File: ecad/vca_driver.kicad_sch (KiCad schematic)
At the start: 7 parts, among them Q2 BD140, Q4 BD139, U3 OPA2277

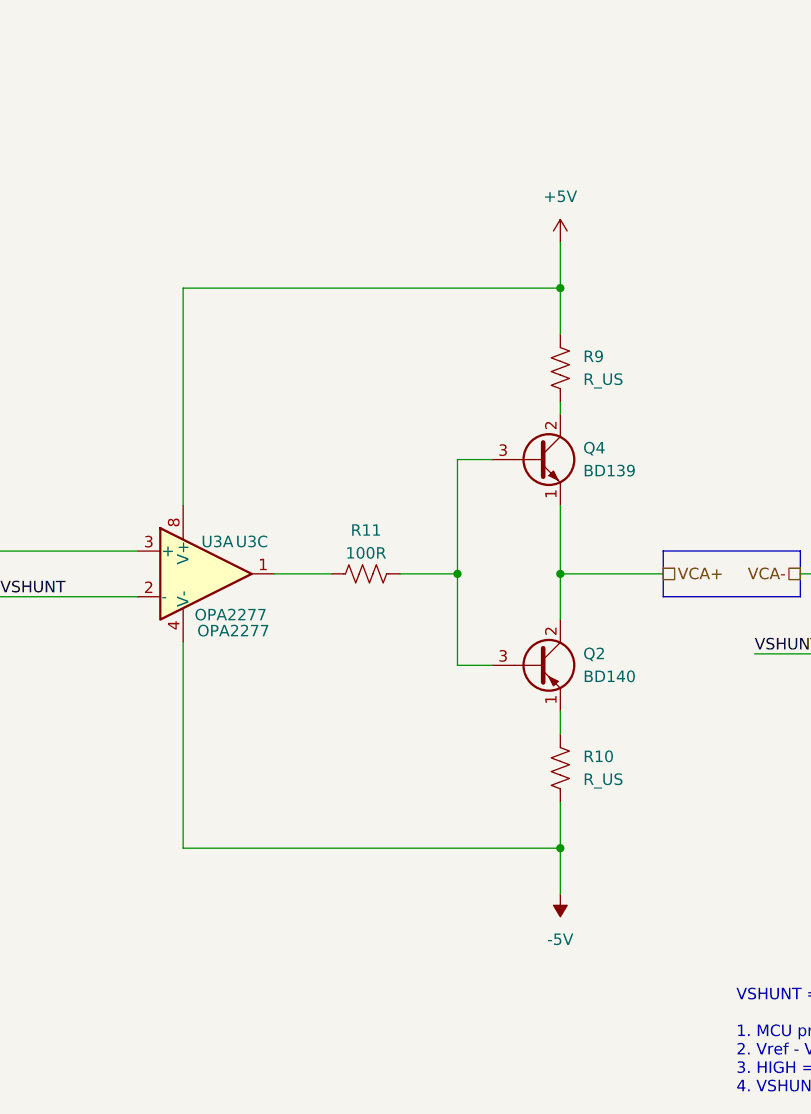
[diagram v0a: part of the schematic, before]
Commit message: more sizing
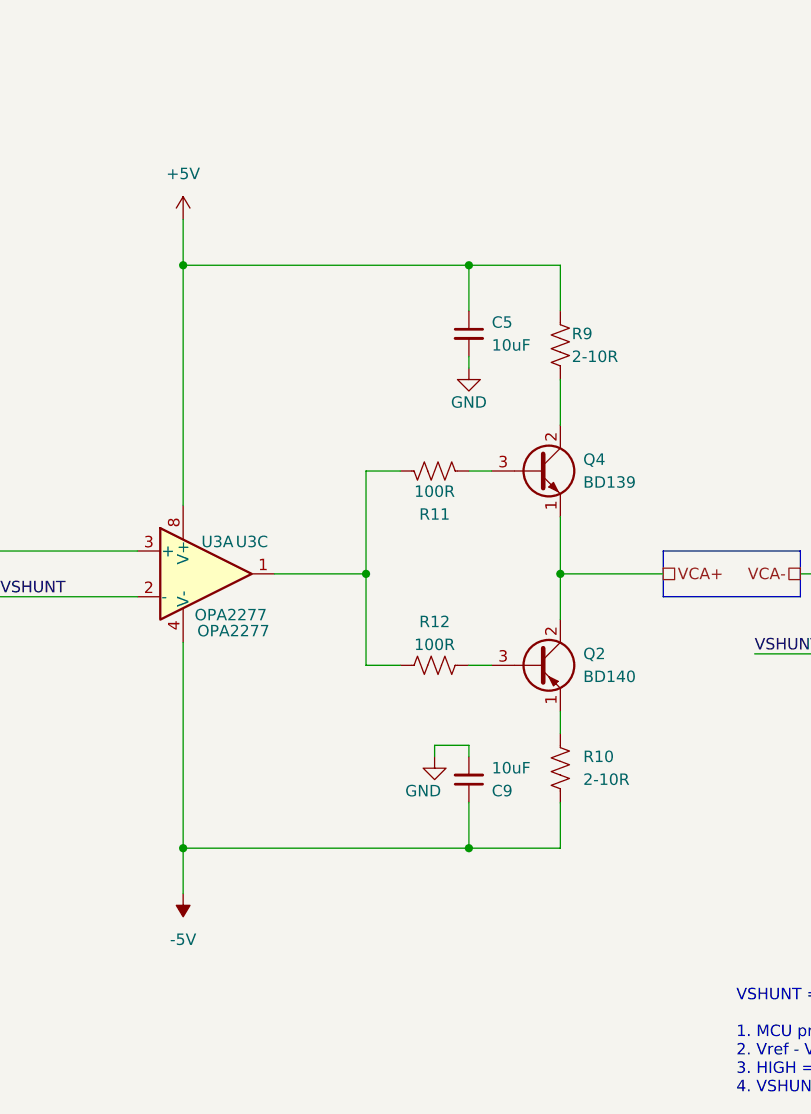
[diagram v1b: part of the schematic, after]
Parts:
- added C5, C9: 10uF, symbol Device:C_Small
- added R12: 100R, symbol Device:R_US
- R10, R9: value R_US -> 2-10R
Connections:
- net +5V: now also C5.1
- net -5V: now also C9.1
- net GND: now also C5.2, C9.2
- net at R11.2, U3.1: now also R12.2
- net at Q4.3 (B), R11.1: no longer Q2.3 (B)
- new net: Q2.3 (B), R12.1
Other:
- moved on the sheet: Q4, R11, R9

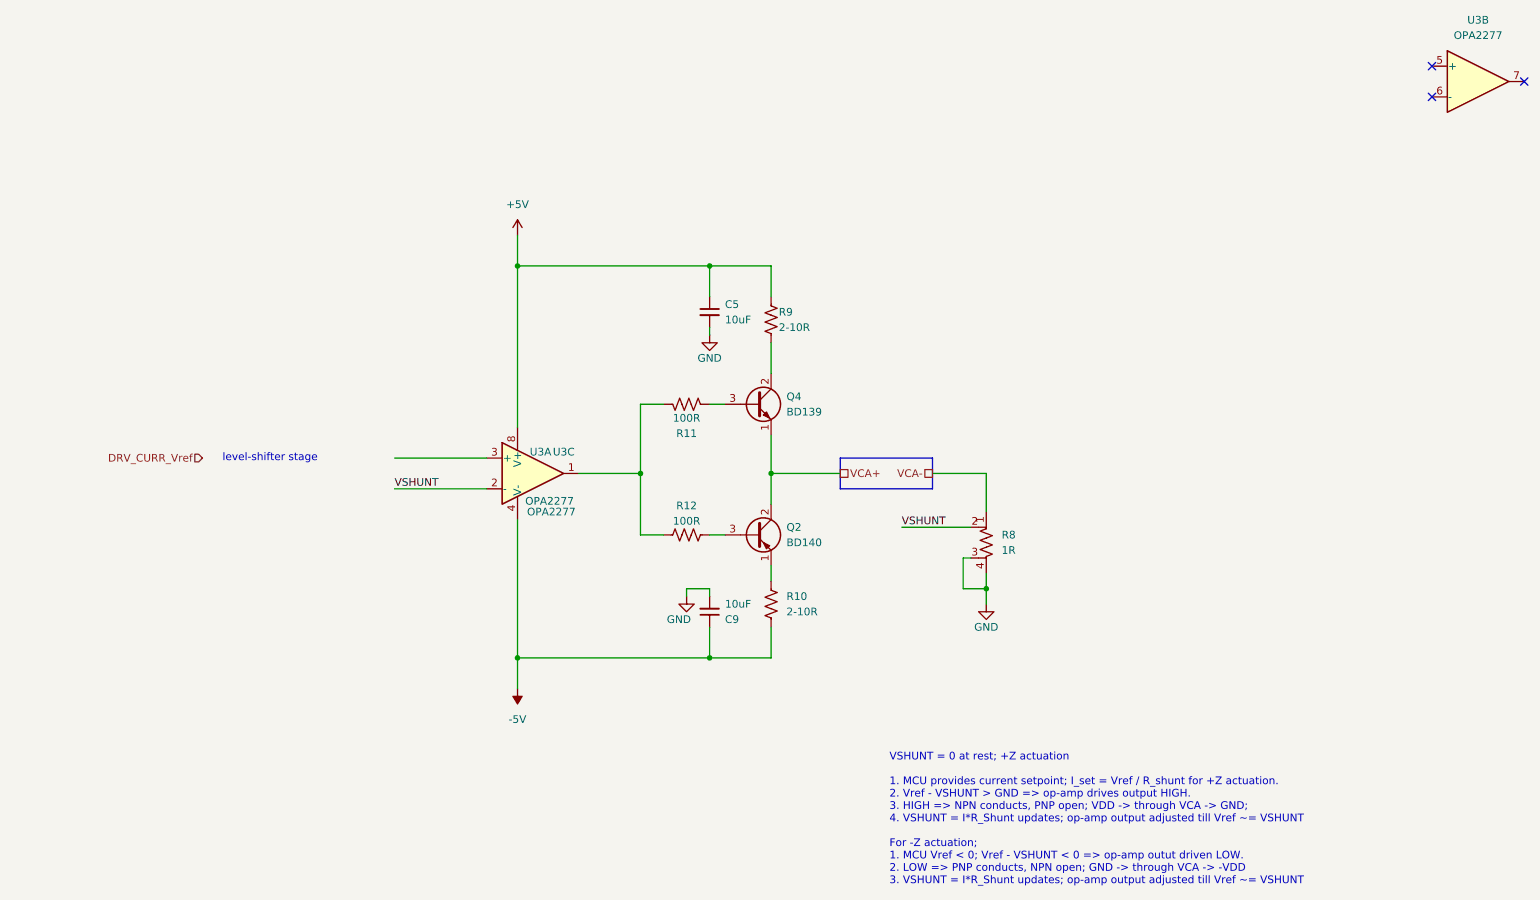
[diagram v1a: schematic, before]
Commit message: pp
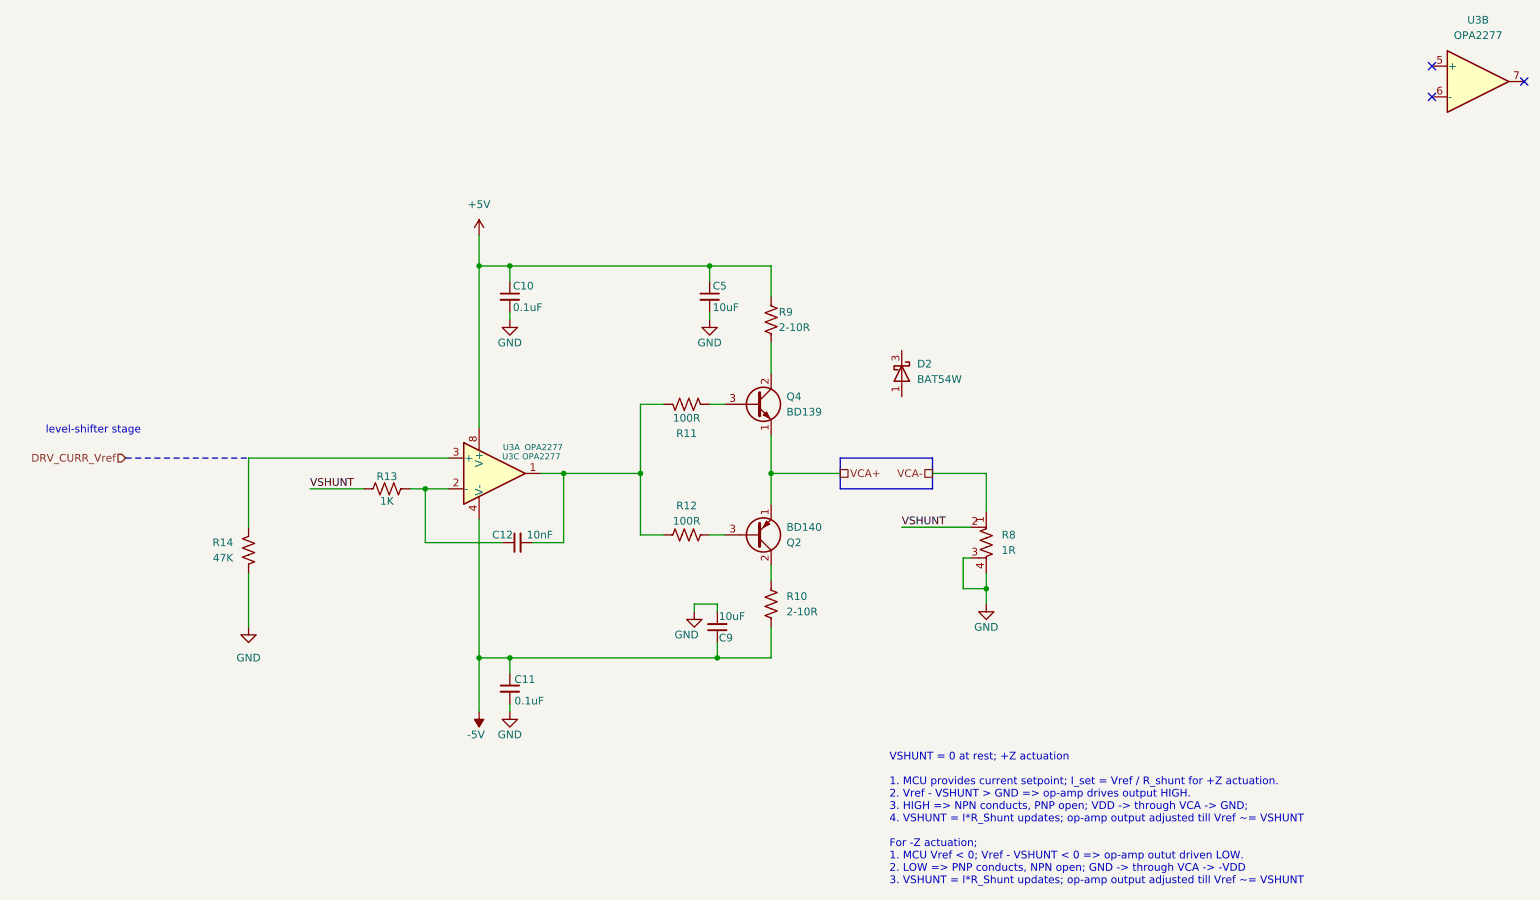
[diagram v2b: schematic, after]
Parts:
- added C10, C11: 0.1uF, symbol Device:C_Small
- added C12: 10nF, symbol Device:C_Small
- added D2: BAT54W, Package_TO_SOT_SMD:SOT-323_SC-70, symbol Diode:BAT54W
- added R13: 1K, symbol Device:R_US
- added R14: 47K, symbol Device:R_US
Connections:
- net +5V: now also C10.1
- net -5V: now also C11.1
- net GND: now also C10.2, C11.2, R14.2
- net VCA+: now also Q2.1 (E); no longer Q2.2 (C)
- net VSHUNT: now also R13.1; no longer U3.2 (-)
- net at R11.2, R12.2, U3.1: now also C12.2
- net at U3.3 (+): now also R14.1
- net at R10.1: now also Q2.2 (C); no longer Q2.1 (E)
- new net: C12.1, R13.2, U3.2 (-)
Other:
- moved on the sheet: C5, C9, U3A, U3C
